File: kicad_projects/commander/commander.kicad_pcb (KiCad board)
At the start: 2 copper layers, 50 x 70 mm, 18 parts, among them J1 left input IDC14, J2 right input IDC14, J4 TPS pinout, J5 DS1020-12-6VBT1A-R, J6 PSP 3000 connector SFV4R-4STB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, J7 PSP 2000 raw pins out, J8 debug out, Q1 MMFTP3401, SW1 RESET_SWITCH, U1 Pico

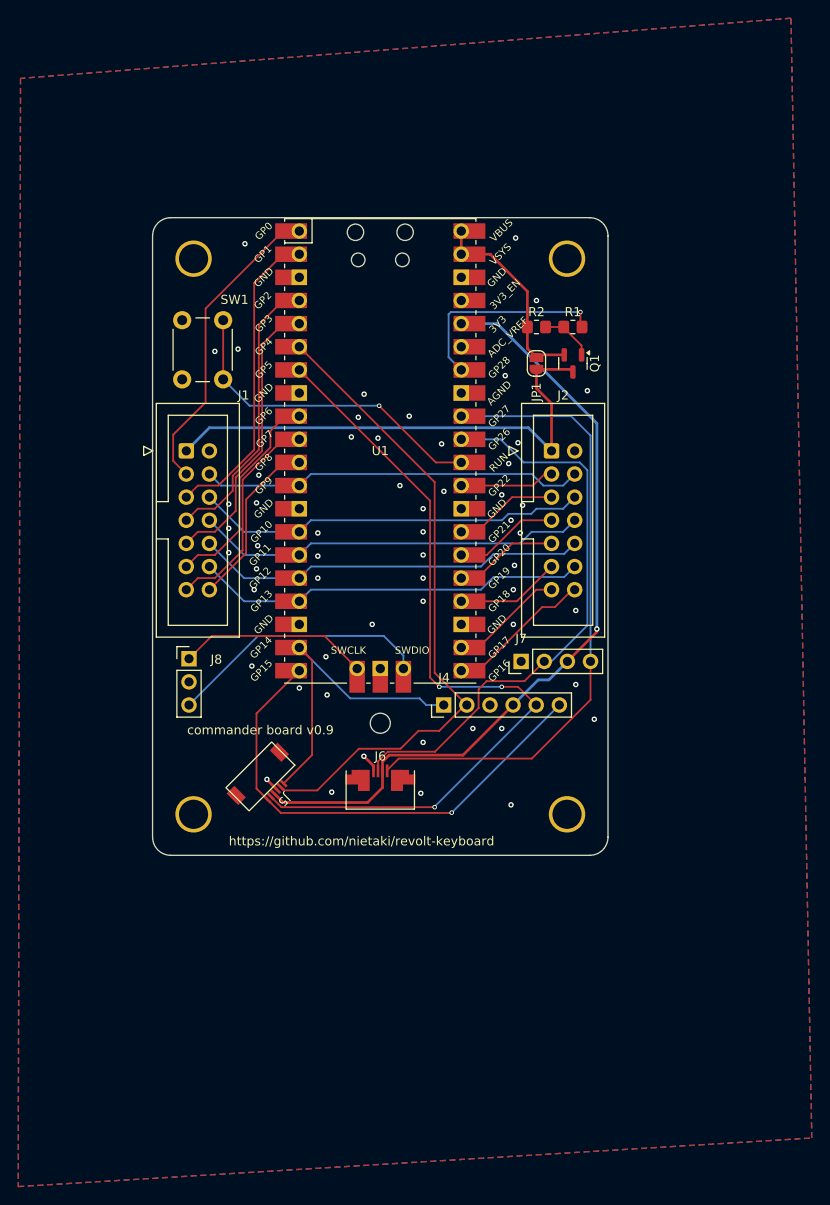
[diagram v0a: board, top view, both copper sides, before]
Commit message: big commander WIP
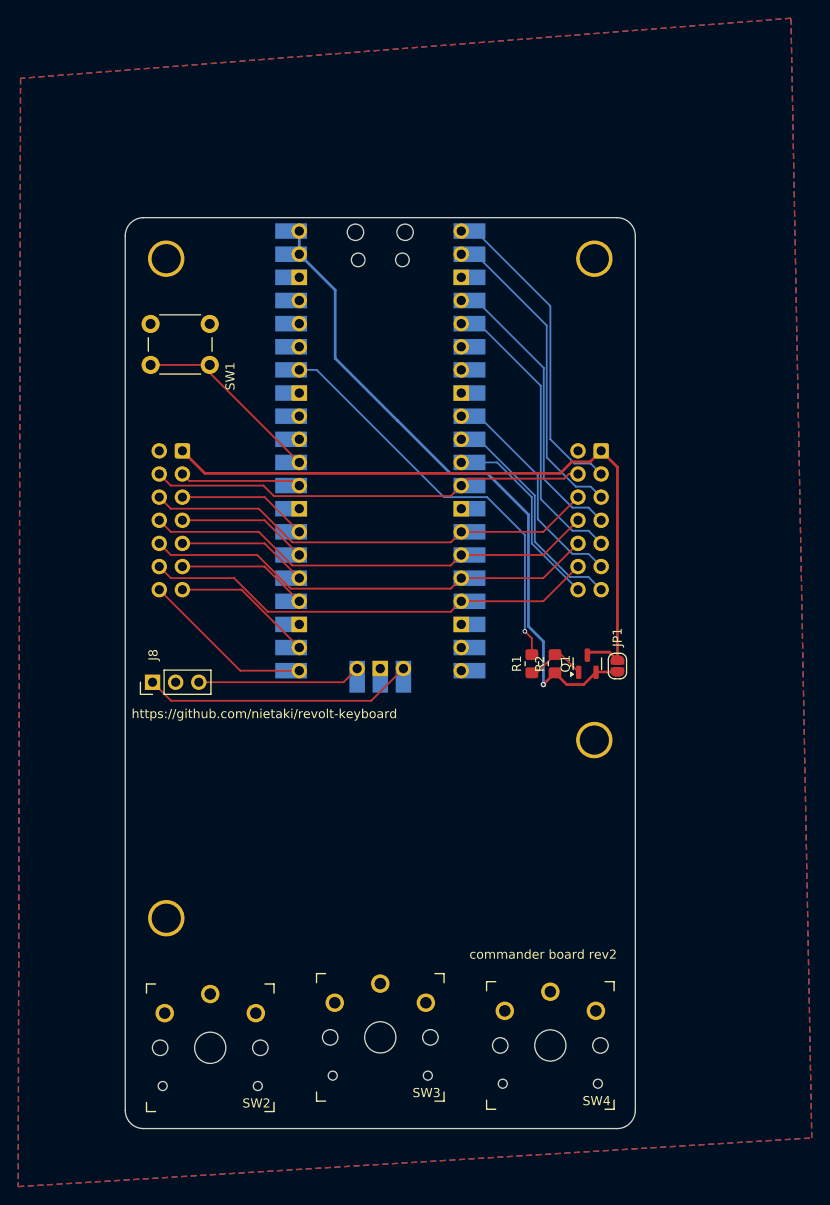
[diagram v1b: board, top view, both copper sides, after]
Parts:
- removed J4: TPS pinout, Connector_PinHeader_2.54mm:PinHeader_1x06_P2.54mm_Vertical
- removed J5: DS1020-12-6VBT1A-R, revolt_footprints:DS1020-12-6VBT1A-R
- removed J6: PSP 3000 connector SFV4R-4STBE1HLF, revolt_footprints:SFV4R-3STBE1HLF
- removed J7: PSP 2000 raw pins out, Connector_PinHeader_2.54mm:PinHeader_1x04_P2.54mm_Vertical
- removed REF**: MountingHole_2.2mm_M2, MountingHole:MountingHole_2.2mm_M2
- added SW2: SW_Push, revolt_footprints:SW_PG1350_reversible_with_keycap_outline, F.Cu at (116.3, 151.1)
- added SW3: SW_Push, revolt_footprints:SW_PG1350_reversible_with_keycap_outline, F.Cu at (135.0, 150.0)
- added SW4: SW_Push, revolt_footprints:SW_PG1350_reversible_with_keycap_outline, F.Cu at (153.7, 150.9)
- J1: value left input IDC14 -> right input IDC14; moved to B.Cu
- J2: value right input IDC14 -> left input IDC14; moved to B.Cu
- U1: moved to B.Cu
- moved J1 45.5 mm to (159.2, 85.6), turned to 180 degrees
- moved J2 40.5 mm to (113.3, 85.6), turned to 180 degrees
- moved R1 37.2 mm to (151.6, 109.0), turned to 90 degrees
- moved R2 37.0 mm to (154.2, 109.0), turned to 90 degrees
- moved JP1 34.4 mm to (161.0, 109.2), turned to 90 degrees
- moved Q1 33.0 mm to (157.7, 109.0), turned to 90 degrees
- moved HOLE_M3 11.8 mm to (111.5, 136.9)
- moved HOLE_M3 8.69 mm to (158.5, 117.3)
- moved SW1 7.01 mm to (109.8, 71.7), turned to 0 degrees
- moved J8 4.76 mm to (110.0, 111.0), turned to 90 degrees
- moved HOLE_M3 3.00 mm to (158.5, 64.5)
- moved HOLE_M3 3.00 mm to (111.5, 64.5)
- turned U1 to 180 degrees
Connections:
- U1 pad 19: /TPS_RDY -> unconnected-(U1-GPIO14-Pad19)
- U1 pad 20: /TPS_NRST -> unconnected-(U1-GPIO15-Pad20)
- U1 pad 6: /TPS_SDA -> unconnected-(U1-GPIO4-Pad6)
- U1 pad 7: /TPS_SCL -> unconnected-(U1-GPIO5-Pad7)
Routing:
- net 3V3: track 87.6 -> 0.00 mm, vias 1 -> 0
- net /TPS_SCL: track 87.0 -> 0.00 mm, vias 3 -> 0
- net /TPS_SDA: track 71.5 -> 0.00 mm
- net /X2: track 70.5 -> 0.00 mm
- net /X1: track 64.0 -> 0.00 mm
- net /TPS_NRST: track 54.2 -> 0.00 mm, vias 1 -> 0
- net 5V: track 24.2 -> 73.0 mm, vias 0 -> 1
- net /TPS_RDY: track 35.3 -> 0.00 mm
- net /NOT_LED_ENABLE: track 23.0 -> 45.7 mm
- net LED_5V: track 56.0 -> 75.5 mm
- net /RUN: track 36.4 -> 21.3 mm, vias 1 -> 0
- net Net-(J8-Pin_3): track 29.0 -> 18.0 mm
- net Net-(J8-Pin_1): track 21.0 -> 29.8 mm
- net /ROW3: track 43.3 -> 50.1 mm
- net /ROW1: track 43.3 -> 50.1 mm
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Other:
- board size 50 x 70 mm -> 56 x 100 mm
- board text added: "commander board rev2"
- board text removed: "PSP joystick"
- board text removed: "TPS43"
- board text removed: "commander board v0.9"
